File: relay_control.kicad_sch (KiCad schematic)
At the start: 12 parts

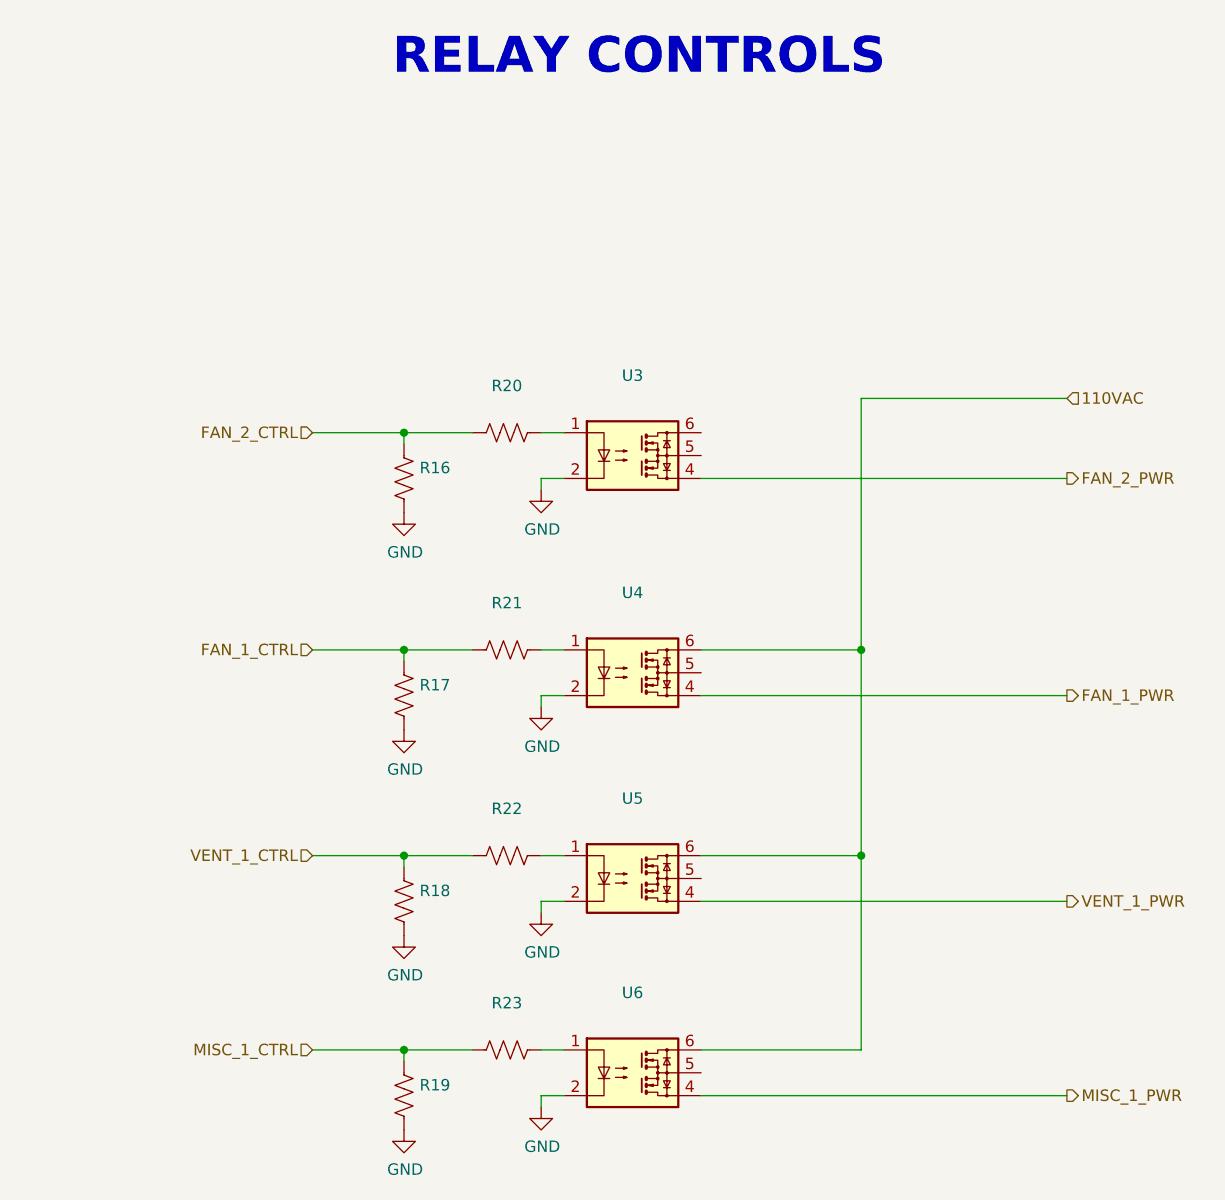
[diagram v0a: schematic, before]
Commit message: Continued with layout.
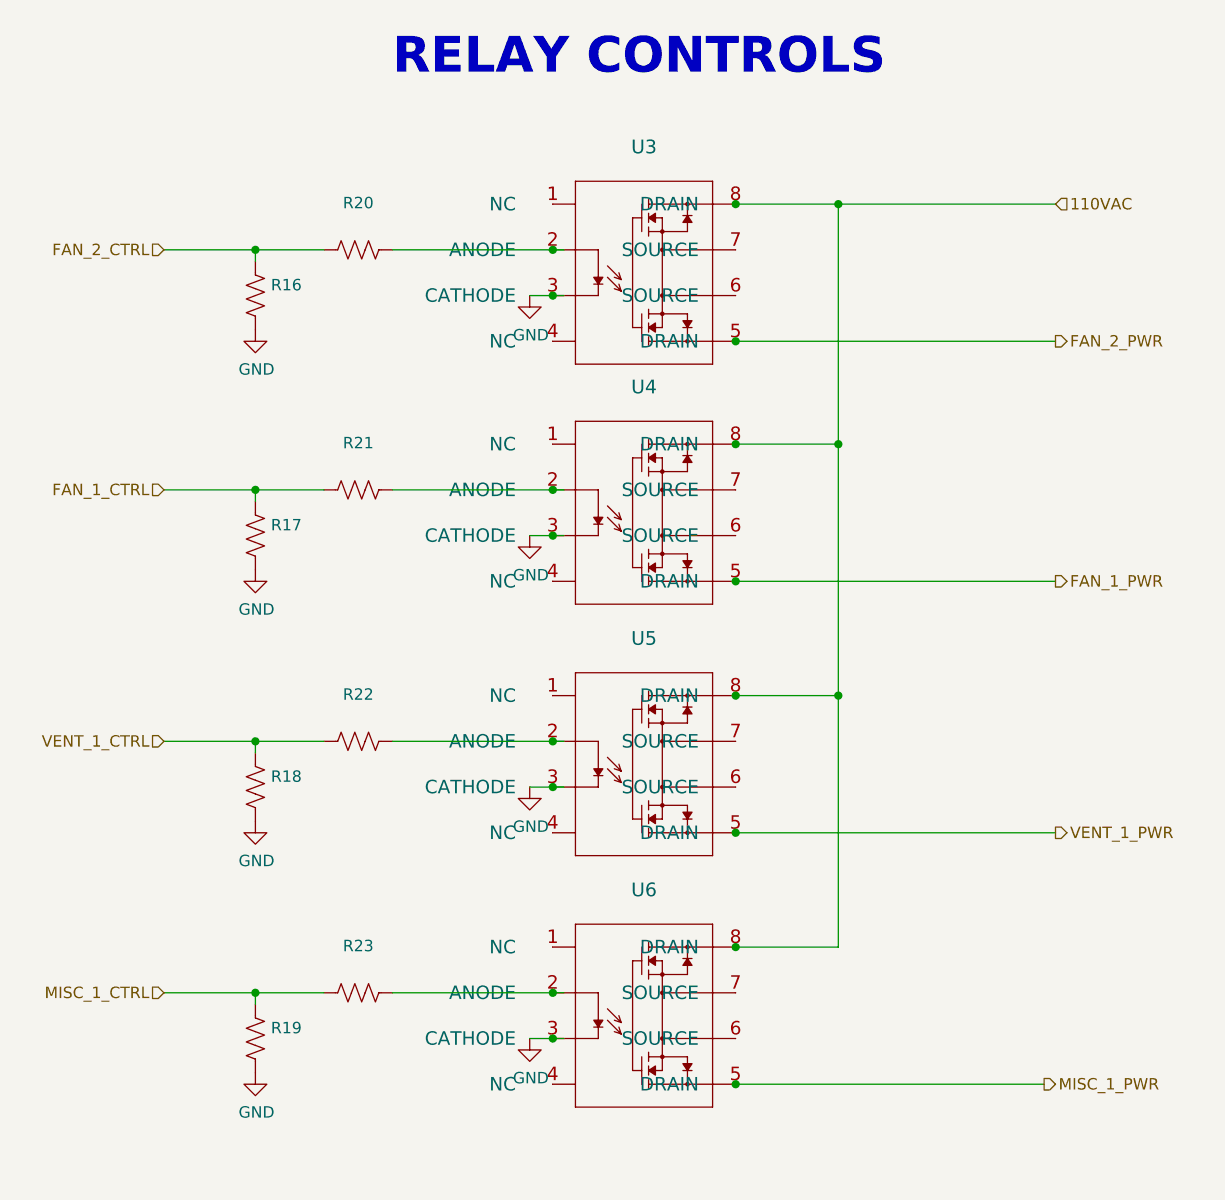
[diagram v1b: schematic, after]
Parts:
- removed U3, U4, U5, U6: (no value), symbol Relay_SolidState:TLP3546
- added U3, U4, U5, U6: (no value), symbol TLP3825:TLP3825TP1_F
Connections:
- net 110VAC: now also U3.8 (DRAIN), U4.8 (DRAIN), U5.8 (DRAIN), U6.8 (DRAIN)
- net FAN_1_PWR: now also U4.5 (DRAIN)
- net FAN_2_PWR: now also U3.5 (DRAIN)
- net GND: now also U3.3 (CATHODE), U4.3 (CATHODE), U5.3 (CATHODE), U6.3 (CATHODE)
- net MISC_1_PWR: now also U6.5 (DRAIN)
- net VENT_1_PWR: now also U5.5 (DRAIN)
- net at R21.1: now also U4.2 (ANODE)
- net at R20.1: now also U3.2 (ANODE)
- net at R22.1: now also U5.2 (ANODE)
- net at R23.1: now also U6.2 (ANODE)
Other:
- moved on the sheet: R16, R17, R18, R19, R20, R21, R22, R23
